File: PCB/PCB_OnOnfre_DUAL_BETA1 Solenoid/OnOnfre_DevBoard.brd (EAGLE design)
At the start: 44.1 x 43.8 mm, 32 parts, among them J1 9PIN 2.54MM, J3Y S8050, J7 8p, K1 G5Q-1-DC12, K2 G5Q-1-DC12, U2 esp12

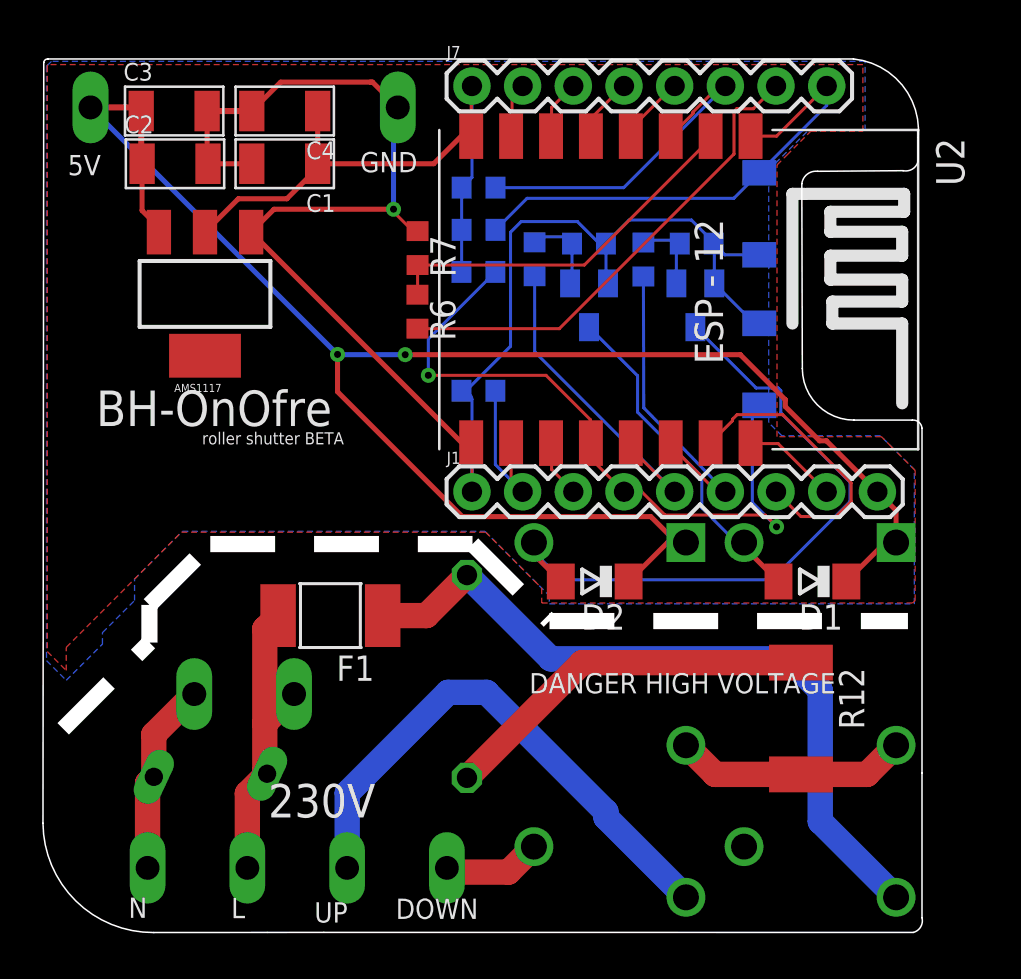
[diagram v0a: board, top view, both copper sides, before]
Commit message: estores rev1
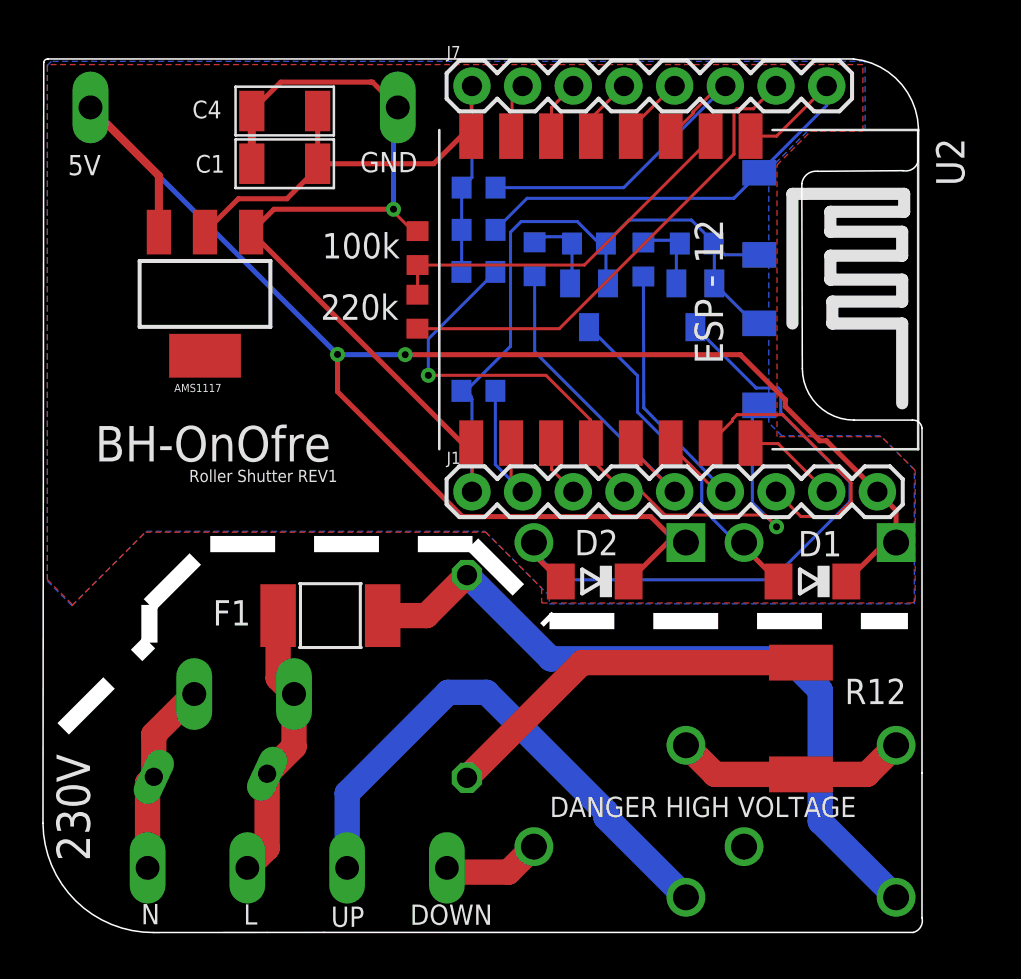
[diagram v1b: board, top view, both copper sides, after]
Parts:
- removed C2, C3: 1NF, Seeed-Capacitor:C1206
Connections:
- net GND: no longer C2.2, C3.2
- net VCC: no longer C2.1, C3.1
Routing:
- net GND: track 84.6 -> 80.1 mm
- net VCC: track 89.7 -> 87.7 mm
- net LINE_L: track 15.5 -> 13.9 mm
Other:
- board text added: "Roller Shutter REV1"
- board text removed: "HLK-PM01"
- board text removed: "L1"
- board text removed: "L2"
- board text removed: "roller shutter BETA"
